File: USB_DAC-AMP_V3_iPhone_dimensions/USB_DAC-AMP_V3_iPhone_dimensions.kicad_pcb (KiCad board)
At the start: 4 copper layers, 70.7 x 188.5 mm, 129 parts, among them J1 USB_C_Receptacle, J2 SJ-3524-SMT, U1 PCM2900C, U10 NE5532, U11 NE5532, U2 TPS61040DBV, U3 SPX3819M5-L, U4 SPX3819M5-L, U5 NE5532, U6 NE5532, U7 NE5532, U8 NE5532, U9 NE5532, Y3 12 MHz Crystal

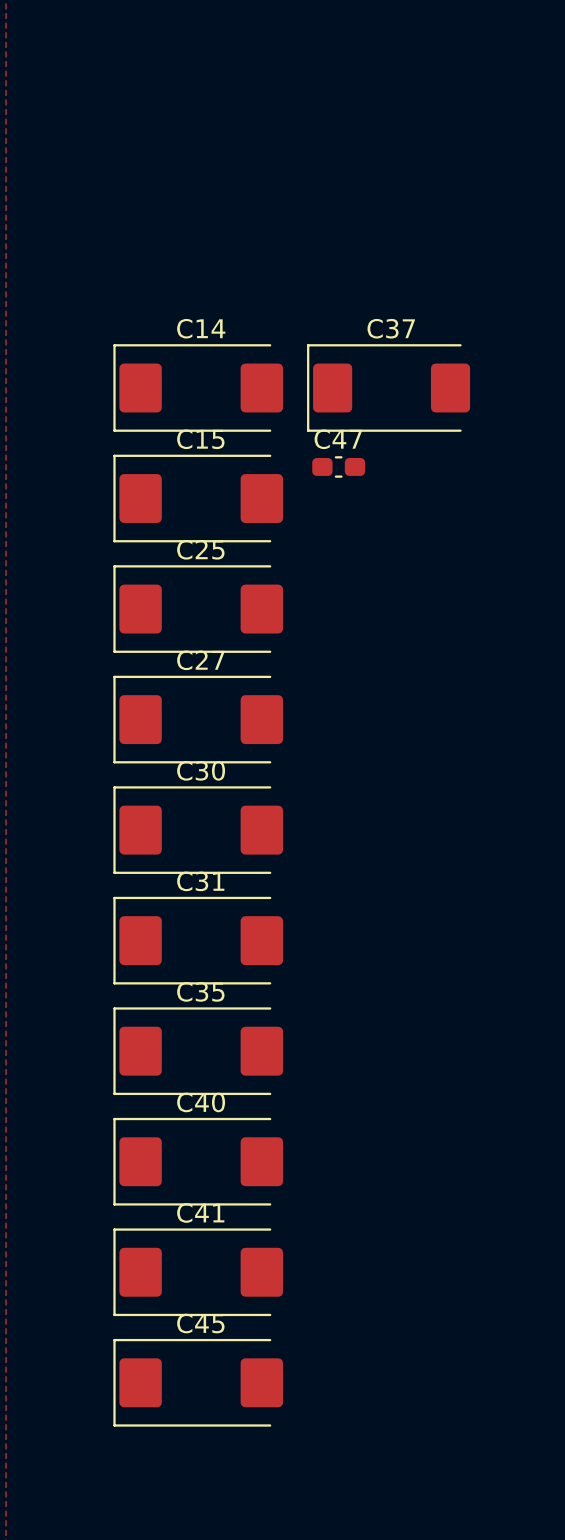
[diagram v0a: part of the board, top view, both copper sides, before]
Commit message: Submitted V1 to Kicad
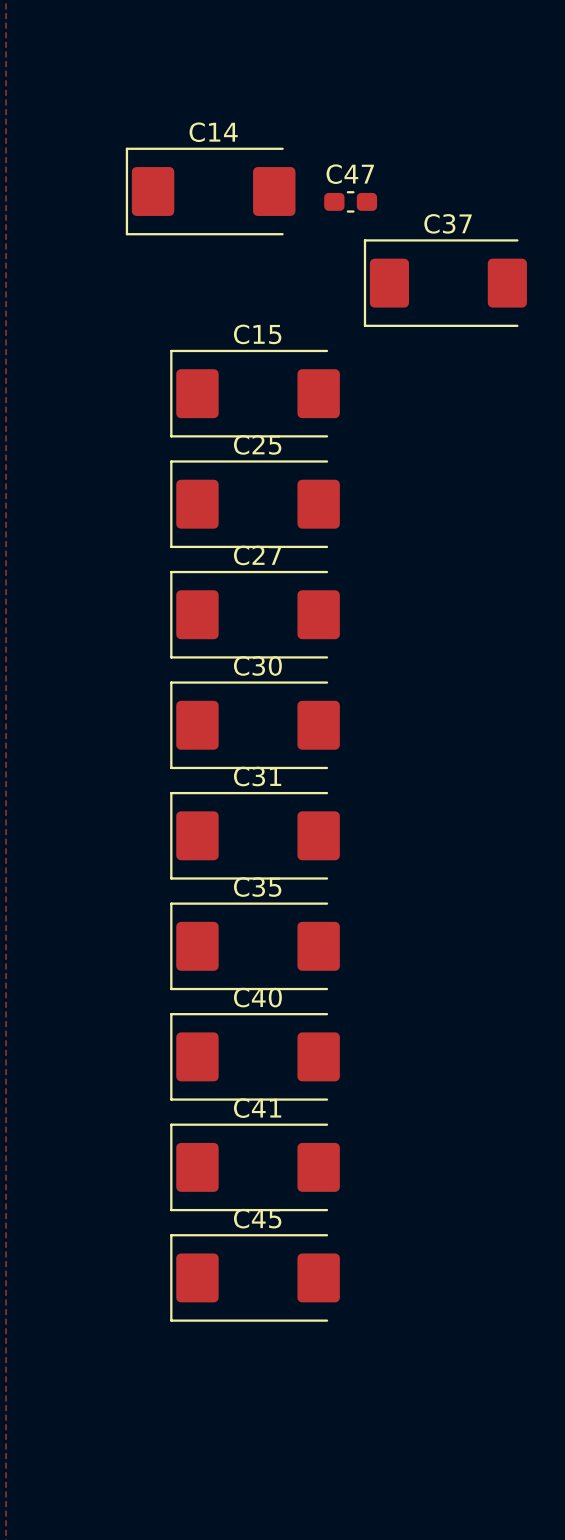
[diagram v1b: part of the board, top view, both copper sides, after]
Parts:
- moved C47 14.0 mm to (222.2, 69.0)
- moved C14 10.4 mm to (214.9, 68.5)
- moved C31 6.31 mm to (217.3, 102.6)
- moved C45 6.31 mm to (217.3, 126.0)
- moved C15 6.31 mm to (217.3, 79.2)
- moved C25 6.31 mm to (217.3, 85.0)
- moved C27 6.31 mm to (217.3, 90.9)
- moved C30 6.31 mm to (217.3, 96.8)
- moved C35 6.31 mm to (217.3, 108.5)
- moved C40 6.31 mm to (217.3, 114.3)
- moved C41 6.31 mm to (217.3, 120.2)
- moved C37 6.31 mm to (227.4, 73.3)
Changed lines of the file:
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@@
 	(footprint "Capacitor_Tantalum_SMD:CP_EIA-7343-43_Kemet-X_HandSolder"
 		(layer "F.Cu")
-		(at 214.2925 119.85)
+		(at 217.3 114.3)
 		(descr "Tantalum Capacitor SMD Kemet-X (7343-43 Metric), IPC-7352 nominal, (Body size from: http://www.kemet.com/Lists/ProductCatalog/Attachments/253/KEM_TC101_STD.pdf), generated with kicad-footprint-generator")
 		(tags "capacitor tantalum")
@@
 	(footprint "Capacitor_Tantalum_SMD:CP_EIA-7343-43_Kemet-X_HandSolder"
 		(layer "F.Cu")
-		(at 214.2925 90.6)
+		(at 217.3 85.05)
 		(descr "Tantalum Capacitor SMD Kemet-X (7343-43 Metric), IPC-7352 nominal, (Body size from: http://www.kemet.com/Lists/ProductCatalog/Attachments/253/KEM_TC101_STD.pdf), generated with kicad-footprint-generator")
 		(tags "capacitor tantalum")
@@
 	(footprint "Capacitor_Tantalum_SMD:CP_EIA-7343-43_Kemet-X_HandSolder"
 		(layer "F.Cu")
-		(at 214.2925 96.45)
+		(at 217.3 90.9)
 		(descr "Tantalum Capacitor SMD Kemet-X (7343-43 Metric), IPC-7352 nominal, (Body size from: http://www.kemet.com/Lists/ProductCatalog/Attachments/253/KEM_TC101_STD.pdf), generated with kicad-footprint-generator")
 		(tags "capacitor tantalum")
@@
 	(footprint "Capacitor_Tantalum_SMD:CP_EIA-7343-43_Kemet-X_HandSolder"
 		(layer "F.Cu")
-		(at 214.2925 114)
+		(at 217.3 108.45)
 		(descr "Tantalum Capacitor SMD Kemet-X (7343-43 Metric), IPC-7352 nominal, (Body size from: http://www.kemet.com/Lists/ProductCatalog/Attachments/253/KEM_TC101_STD.pdf), generated with kicad-footprint-generator")
 		(tags "capacitor tantalum")
@@
 	(footprint "Capacitor_SMD:C_0603_1608Metric_Pad1.08x0.95mm_HandSolder"
 		(layer "F.Cu")
-		(at 221.5675 83.08)
+		(at 222.2 69.05)
 		(descr "Capacitor SMD 0603 (1608 Metric), square (rectangular) end terminal, IPC-7351 nominal with elongated pad for handsoldering. (Body size source: IPC-SM-782 page 76, https://www.pcb-3d.com/wordpress/wp-content/uploads/ipc-sm-782a_amendment_1_and_2.pdf), generated with kicad-footprint-generator")
 		(tags "capacitor handsolder")
@@
 	(footprint "Capacitor_Tantalum_SMD:CP_EIA-7343-43_Kemet-X_HandSolder"
 		(layer "F.Cu")
-		(at 214.2925 125.7)
+		(at 217.3 120.15)
 		(descr "Tantalum Capacitor SMD Kemet-X (7343-43 Metric), IPC-7352 nominal, (Body size from: http://www.kemet.com/Lists/ProductCatalog/Attachments/253/KEM_TC101_STD.pdf), generated with kicad-footprint-generator")
 		(tags "capacitor tantalum")
@@
 	(footprint "Capacitor_Tantalum_SMD:CP_EIA-7343-43_Kemet-X_HandSolder"
 		(layer "F.Cu")
-		(at 214.2925 84.75)
+		(at 217.3 79.2)
 		(descr "Tantalum Capacitor SMD Kemet-X (7343-43 Metric), IPC-7352 nominal, (Body size from: http://www.kemet.com/Lists/ProductCatalog/Attachments/253/KEM_TC101_STD.pdf), generated with kicad-footprint-generator")
 		(tags "capacitor tantalum")
@@
 	(footprint "Capacitor_Tantalum_SMD:CP_EIA-7343-43_Kemet-X_HandSolder"
 		(layer "F.Cu")
-		(at 214.2925 108.15)
+		(at 217.3 102.6)
 		(descr "Tantalum Capacitor SMD Kemet-X (7343-43 Metric), IPC-7352 nominal, (Body size from: http://www.kemet.com/Lists/ProductCatalog/Attachments/253/KEM_TC101_STD.pdf), generated with kicad-footprint-generator")
 		(tags "capacitor tantalum")
@@
 	(footprint "Capacitor_Tantalum_SMD:CP_EIA-7343-43_Kemet-X_HandSolder"
 		(layer "F.Cu")
-		(at 214.2925 102.3)
+		(at 217.3 96.75)
 		(descr "Tantalum Capacitor SMD Kemet-X (7343-43 Metric), IPC-7352 nominal, (Body size from: http://www.kemet.com/Lists/ProductCatalog/Attachments/253/KEM_TC101_STD.pdf), generated with kicad-footprint-generator")
 		(tags "capacitor tantalum")
@@
 	(footprint "Capacitor_Tantalum_SMD:CP_EIA-7343-43_Kemet-X_HandSolder"
 		(layer "F.Cu")
-		(at 214.2925 78.9)
+		(at 214.95 68.5)
 		(descr "Tantalum Capacitor SMD Kemet-X (7343-43 Metric), IPC-7352 nominal, (Body size from: http://www.kemet.com/Lists/ProductCatalog/Attachments/253/KEM_TC101_STD.pdf), generated with kicad-footprint-generator")
 		(tags "capacitor tantalum")
@@
 	(footprint "Capacitor_Tantalum_SMD:CP_EIA-7343-15_Kemet-W"
 		(layer "F.Cu")
-		(at 224.3675 78.9)
+		(at 227.375 73.35)
 		(descr "Tantalum Capacitor SMD Kemet-W (7343-15 Metric), IPC-7352 nominal, (Body size from: http://www.kemet.com/Lists/ProductCatalog/Attachments/253/KEM_TC101_STD.pdf), generated with kicad-footprint-generator")
 		(tags "capacitor tantalum")
@@
 	(footprint "Capacitor_Tantalum_SMD:CP_EIA-7343-43_Kemet-X_HandSolder"
 		(layer "F.Cu")
-		(at 214.2925 131.55)
+		(at 217.3 126)
 		(descr "Tantalum Capacitor SMD Kemet-X (7343-43 Metric), IPC-7352 nominal, (Body size from: http://www.kemet.com/Lists/ProductCatalog/Attachments/253/KEM_TC101_STD.pdf), generated with kicad-footprint-generator")
 		(tags "capacitor tantalum")
